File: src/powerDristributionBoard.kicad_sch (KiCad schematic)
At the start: 16 parts, among them CN1 XT90_PCB_Mount_Male, CN2 XT30_PCB_Mount_Female, CN3 XT30_PCB_Mount_Female, CN4 XT30_PCB_Mount_Female

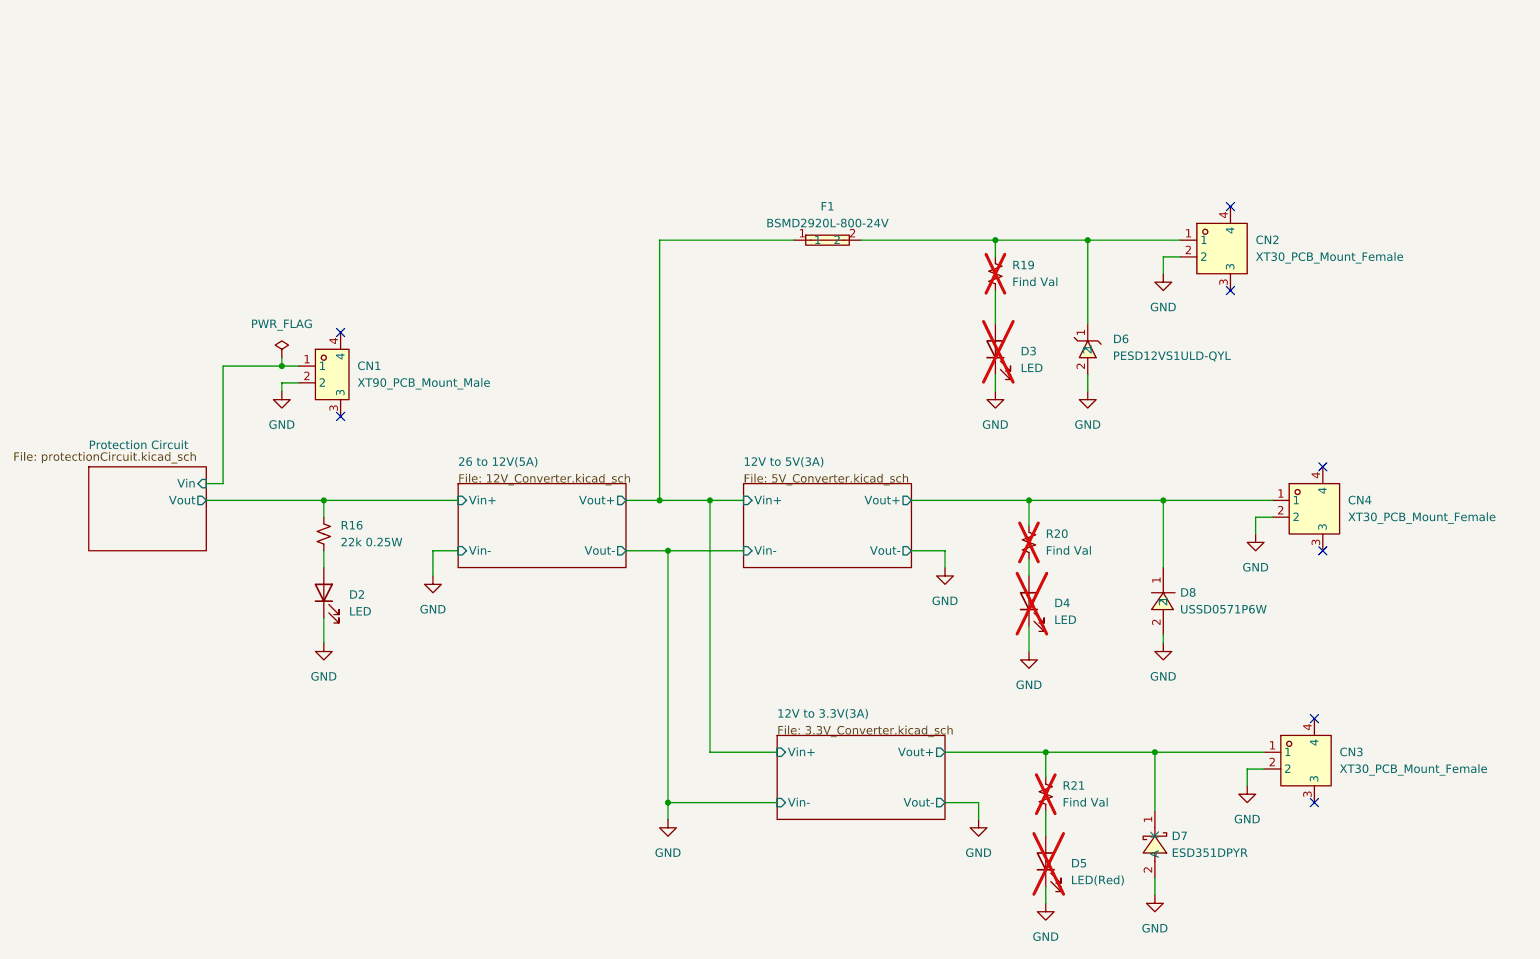
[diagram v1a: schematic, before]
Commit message: GG
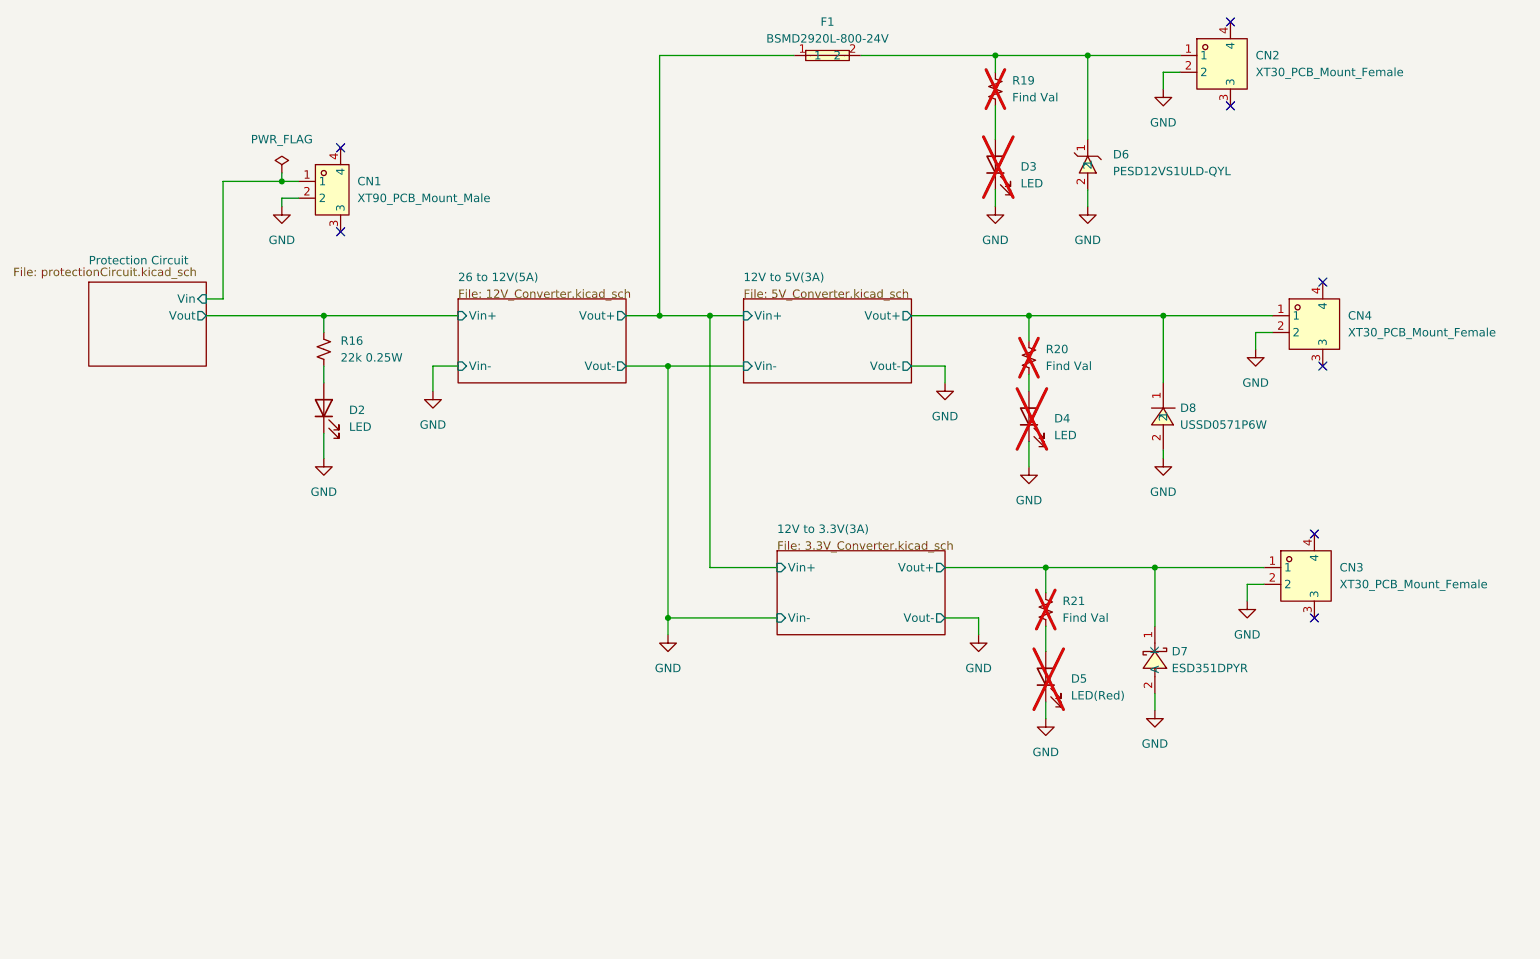
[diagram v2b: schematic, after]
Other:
- moved on the sheet: CN1, CN2, CN3, CN4, D2, D3, D4, D5, D6, D7, D8, F1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
